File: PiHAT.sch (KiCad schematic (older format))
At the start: 28 parts, among them J1 B8B-EH-A, J10 XT30UPB-M, J11 XT30UPB-M, J12 XT30UPB-M, J13 B3B-ZR__LF__SN_, J14 B8B-EH-A, J2 B8B-EH-A, J3 B8B-EH-A, J4 Raspberry_Pi_2_3, J5 B8B-EH-A, J6 B8B-EH-A, J7 XT30UPB-M, J8 XT30UPB-M, J9 XT30UPB-M, U1 74LS151, U2 PCA9685PW, U3 LM2596T-ADJ, U4 74LS151

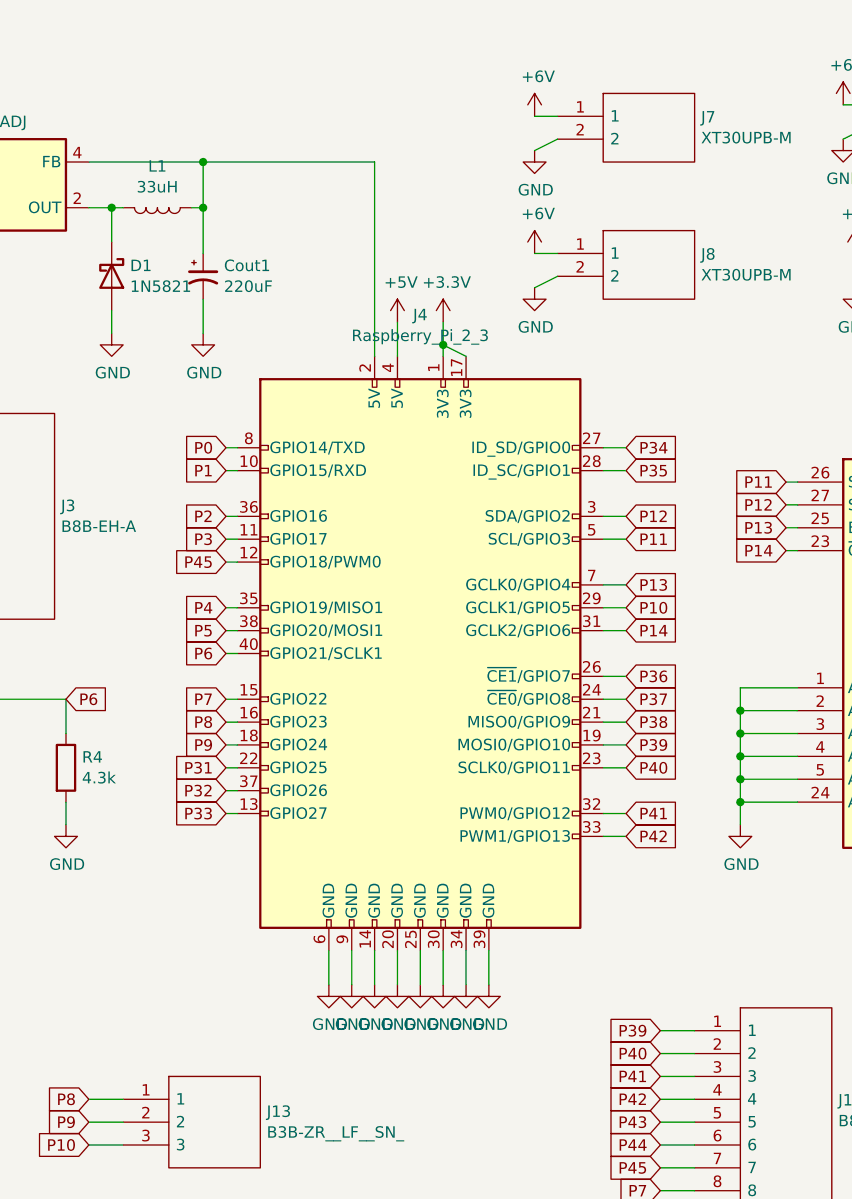
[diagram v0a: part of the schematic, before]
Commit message: Add files via upload
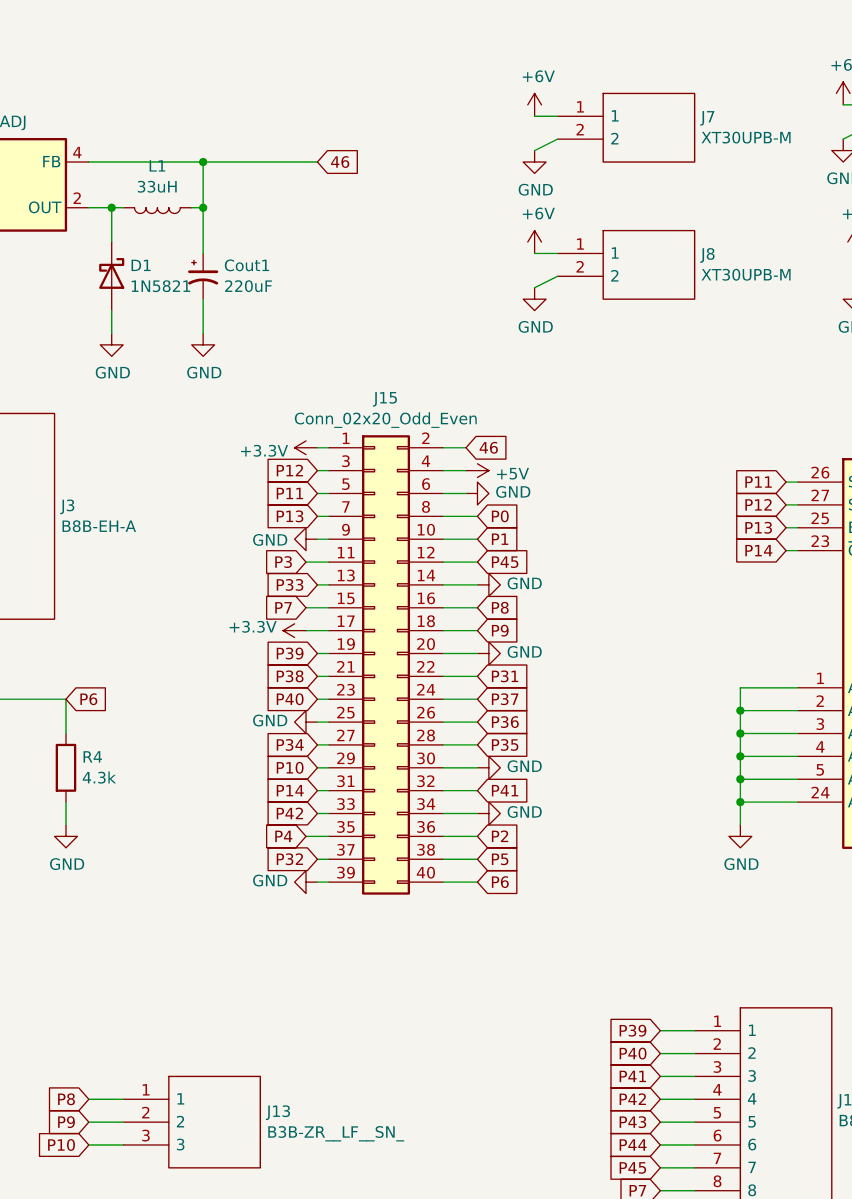
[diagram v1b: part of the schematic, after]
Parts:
- removed J4: Raspberry_Pi_2_3, symbol Connector:Raspberry_Pi_2_3
- added J15: Conn_02x20_Odd_Even, RPi_Hat:Pin_Header_Straight_2x20, symbol Connector_Generic:Conn_02x20_Odd_Even
- Cin1: footprint (none) -> Capacitor_SMD:CP_Elec_4x5.8
- Cout1: footprint (none) -> Capacitor_SMD:CP_Elec_4x5.4
- J1, J14, J2, J3, J5, J6: footprint SHDR8W64P0X250_1X8_2250X380X600P -> SamacSys_Parts:SHDR8W64P0X250_1X8_2250X380X600P
- J10, J11, J12, J7, J8, J9: footprint SHDR2W160P0X500_1X2_1020X520X1070P -> SamacSys_Parts:SHDR2W160P0X500_1X2_1020X520X1070P
- J13: footprint SHDR3W50P0X150_1X3_600X350X450P -> SamacSys_Parts:SHDR3W50P0X150_1X3_600X350X450P
- L1: footprint (none) -> Inductor_SMD:L_12x12mm_H8mm
- R1, R2, R3, R4, R5, R6: footprint (none) -> Resistor_SMD:R_0402_1005Metric
- U1, U4: footprint (none) -> Mux:SOIC127P600X175-16N
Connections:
- net +3V3: now also J15.1 (Pin_1), J15.17 (Pin_17)
- net +5V: now also J15.4 (Pin_4)
- net GND: now also J15.14 (Pin_14), J15.20 (Pin_20), J15.25 (Pin_25), J15.30 (Pin_30), J15.34 (Pin_34), J15.39 (Pin_39), J15.6 (Pin_6), J15.9 (Pin_9)
- net P0: now also J15.8 (Pin_8)
- net P1: now also J15.10 (Pin_10)
- net P10: now also J15.29 (Pin_29)
- net P11: now also J15.5 (Pin_5)
- net P12: now also J15.3 (Pin_3)
- net P13: now also J15.7 (Pin_7)
- net P14: now also J15.31 (Pin_31)
- net P2: now also J15.36 (Pin_36)
- net P3: now also J15.11 (Pin_11)
- net P31: now also J15.22 (Pin_22)
- net P32: now also J15.37 (Pin_37)
- net P33: now also J15.13 (Pin_13)
- net P34: now also J15.27 (Pin_27)
- net P35: now also J15.28 (Pin_28)
- net P36: now also J15.26 (Pin_26)
- net P37: now also J15.24 (Pin_24)
- net P38: now also J15.21 (Pin_21)
- net P39: now also J15.19 (Pin_19)
- net P4: now also J15.35 (Pin_35)
- net P40: now also J15.23 (Pin_23)
- net P41: now also J15.32 (Pin_32)
- net P42: now also J15.33 (Pin_33)
- net P45: now also J15.12 (Pin_12)
- net P5: now also J15.38 (Pin_38)
- net P6: now also J15.40 (Pin_40)
- net P7: now also J15.15 (Pin_15)
- net P8: now also J15.16 (Pin_16)
- net P9: now also J15.18 (Pin_18)
- net 46: now reaches Cout1.1, L1.1, U3.4 (FB)
- net 46: now also J15.2 (Pin_2)

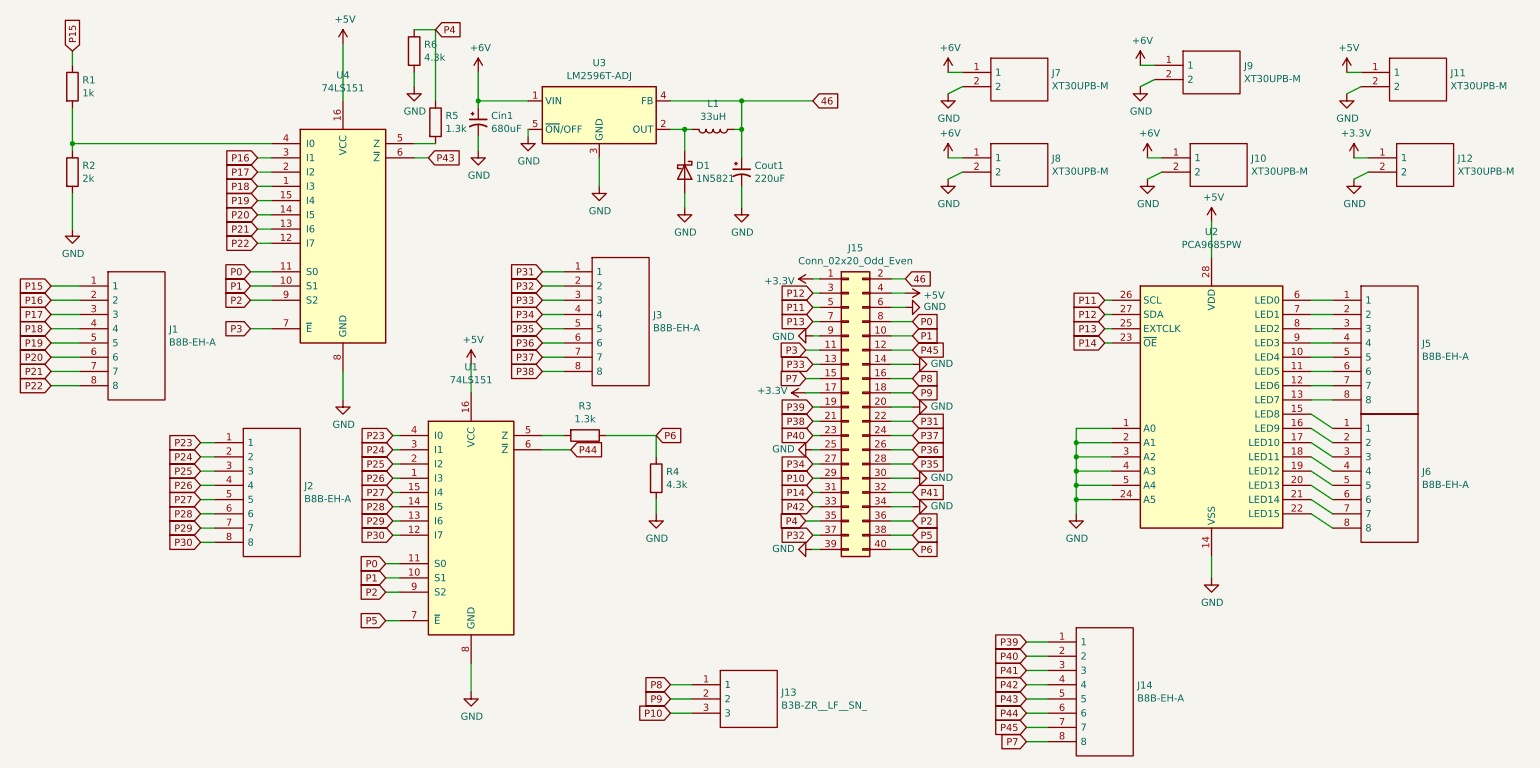
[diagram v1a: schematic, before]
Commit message: Add files via upload
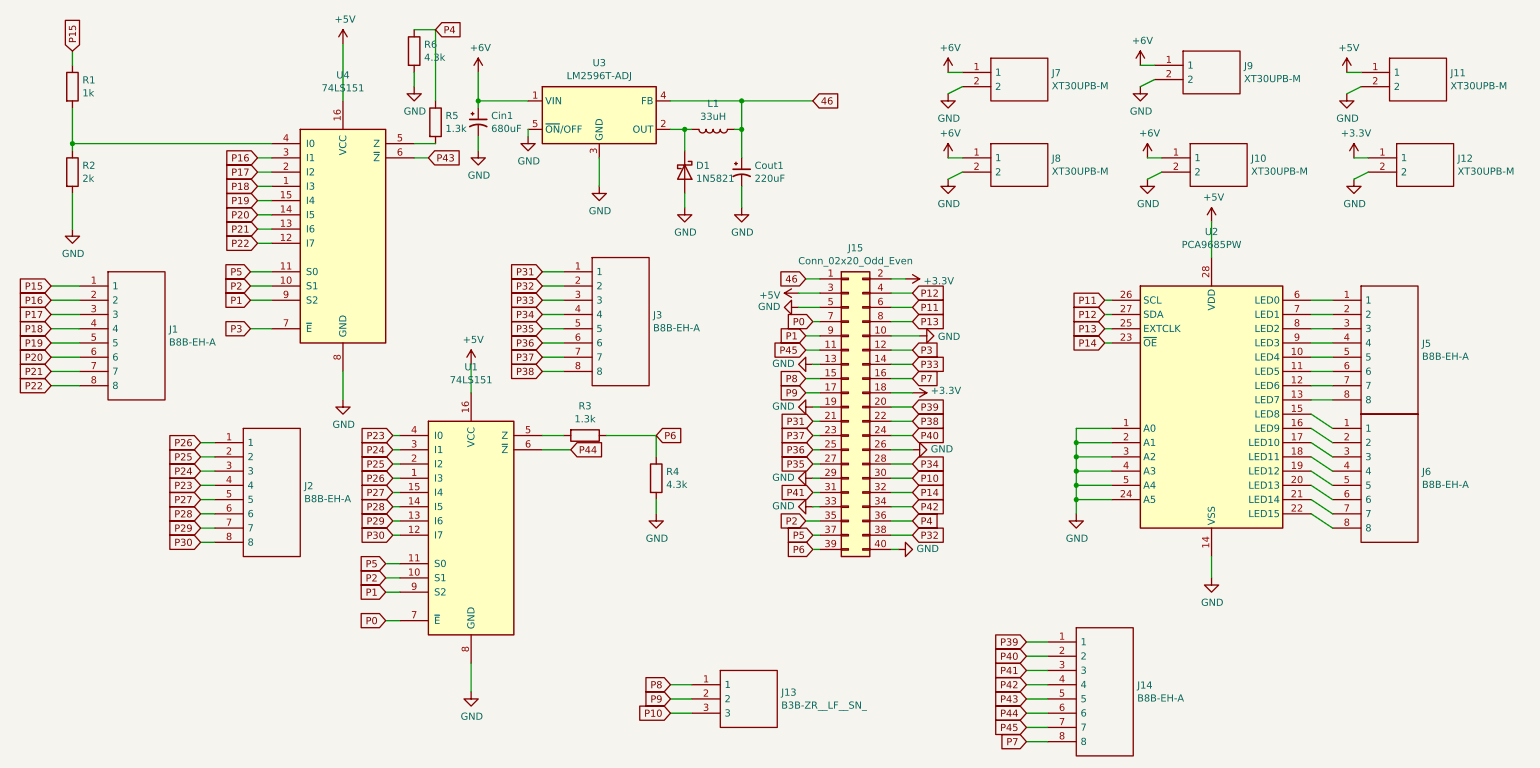
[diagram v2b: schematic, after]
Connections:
- net +3V3: now also J15.18 (Pin_18), J15.2 (Pin_2); no longer J15.1 (Pin_1), J15.17 (Pin_17)
- net +5V: now also J15.3 (Pin_3); no longer J15.4 (Pin_4)
- net 46: now also J15.1 (Pin_1); no longer J15.2 (Pin_2)
- net GND: now also J15.10 (Pin_10), J15.13 (Pin_13), J15.19 (Pin_19), J15.26 (Pin_26), J15.29 (Pin_29), J15.33 (Pin_33), J15.40 (Pin_40), J15.5 (Pin_5); no longer J15.14 (Pin_14), J15.20 (Pin_20), J15.25 (Pin_25), J15.30 (Pin_30), J15.34 (Pin_34), J15.39 (Pin_39), J15.6 (Pin_6), J15.9 (Pin_9)
- net P0: now also J15.7 (Pin_7), U1.7 (~E); no longer J15.8 (Pin_8), U1.11 (S0), U4.11 (S0)
- net P1: now also J15.9 (Pin_9), U1.9 (S2), U4.9 (S2); no longer J15.10 (Pin_10), U1.10 (S1), U4.10 (S1)
- net P10: now also J15.30 (Pin_30); no longer J15.29 (Pin_29)
- net P11: now also J15.6 (Pin_6); no longer J15.5 (Pin_5)
- net P12: now also J15.4 (Pin_4); no longer J15.3 (Pin_3)
- net P13: now also J15.8 (Pin_8); no longer J15.7 (Pin_7)
- net P14: now also J15.32 (Pin_32); no longer J15.31 (Pin_31)
- net P2: now also J15.35 (Pin_35), U1.10 (S1), U4.10 (S1); no longer J15.36 (Pin_36), U1.9 (S2), U4.9 (S2)
- net P23: now also J2.4; no longer J2.1
- net P24: now also J2.3; no longer J2.2
- net P25: now also J2.2; no longer J2.3
- net P26: now also J2.1; no longer J2.4
- net P3: now also J15.12 (Pin_12); no longer J15.11 (Pin_11)
- net P31: now also J15.21 (Pin_21); no longer J15.22 (Pin_22)
- net P32: now also J15.38 (Pin_38); no longer J15.37 (Pin_37)
- net P33: now also J15.14 (Pin_14); no longer J15.13 (Pin_13)
- net P34: now also J15.28 (Pin_28); no longer J15.27 (Pin_27)
- net P35: now also J15.27 (Pin_27); no longer J15.28 (Pin_28)
- net P36: now also J15.25 (Pin_25); no longer J15.26 (Pin_26)
- net P37: now also J15.23 (Pin_23); no longer J15.24 (Pin_24)
- net P38: now also J15.22 (Pin_22); no longer J15.21 (Pin_21)
- net P39: now also J15.20 (Pin_20); no longer J15.19 (Pin_19)
- net P4: now also J15.36 (Pin_36); no longer J15.35 (Pin_35)
- net P40: now also J15.24 (Pin_24); no longer J15.23 (Pin_23)
- net P41: now also J15.31 (Pin_31); no longer J15.32 (Pin_32)
- net P42: now also J15.34 (Pin_34); no longer J15.33 (Pin_33)
- net P45: now also J15.11 (Pin_11); no longer J15.12 (Pin_12)
- net P5: now also J15.37 (Pin_37), U1.11 (S0), U4.11 (S0); no longer J15.38 (Pin_38), U1.7 (~E)
- net P6: now also J15.39 (Pin_39); no longer J15.40 (Pin_40)
- net P7: now also J15.16 (Pin_16); no longer J15.15 (Pin_15)
- net P8: now also J15.15 (Pin_15); no longer J15.16 (Pin_16)
- net P9: now also J15.17 (Pin_17); no longer J15.18 (Pin_18)
